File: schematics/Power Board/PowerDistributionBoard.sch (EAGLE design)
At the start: 11 parts

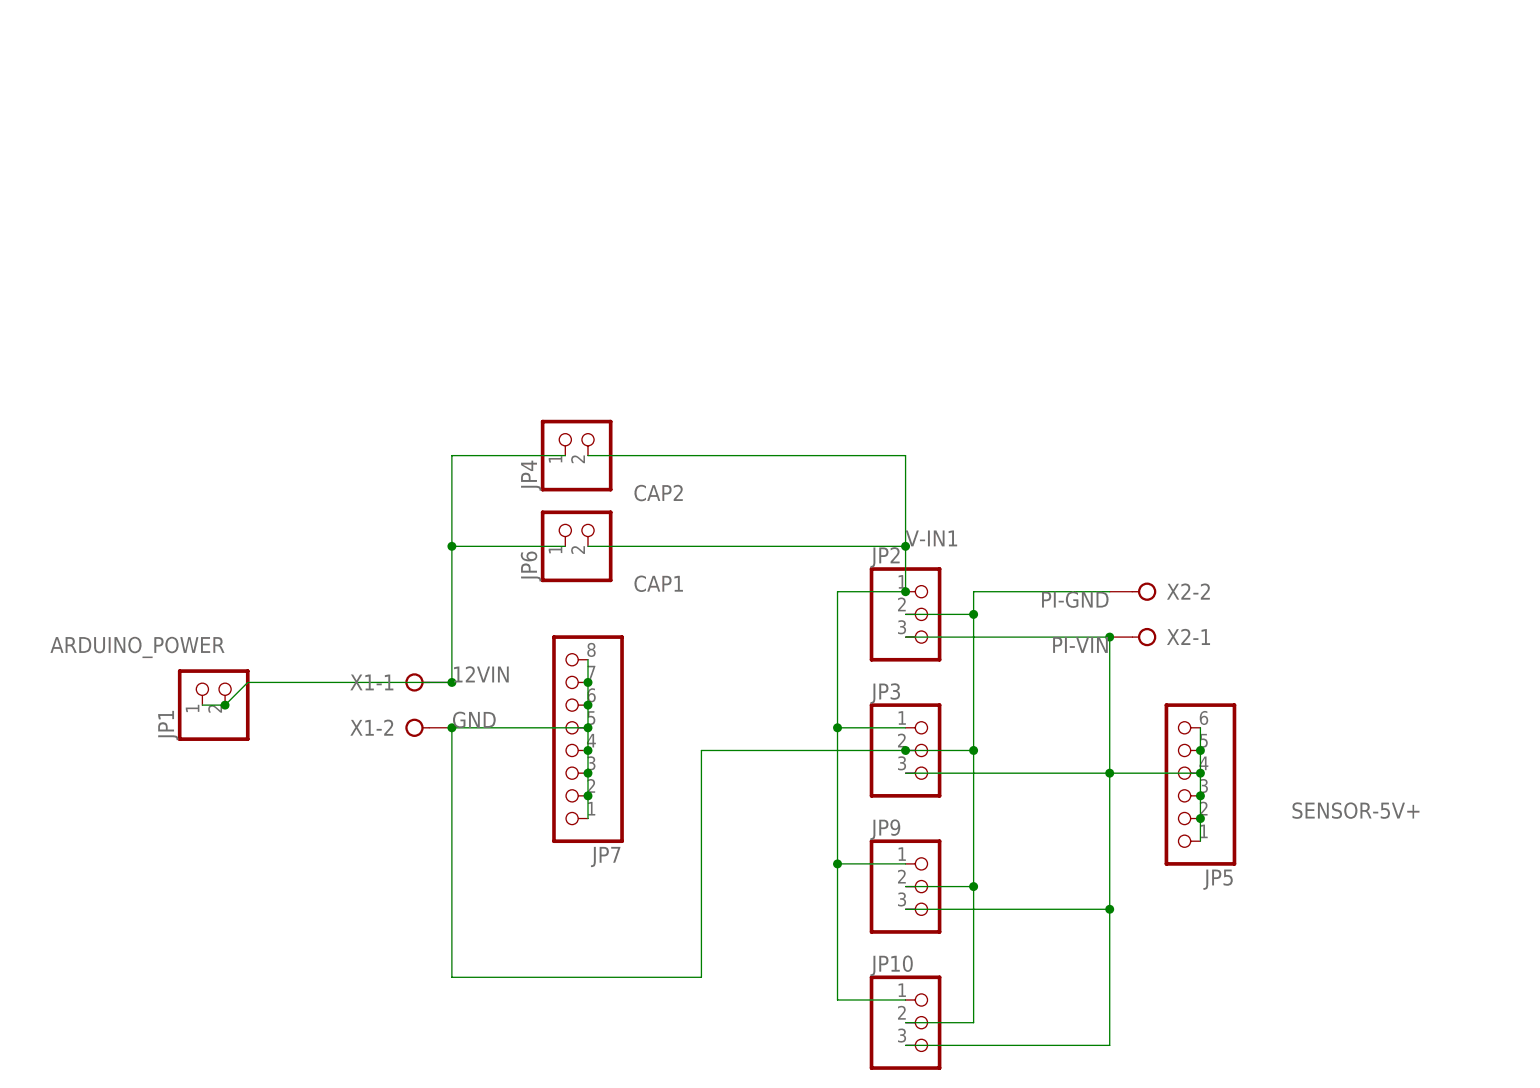
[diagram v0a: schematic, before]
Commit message: Updated Most Recent PCB's
Changed both directories with the most up to date schematics.
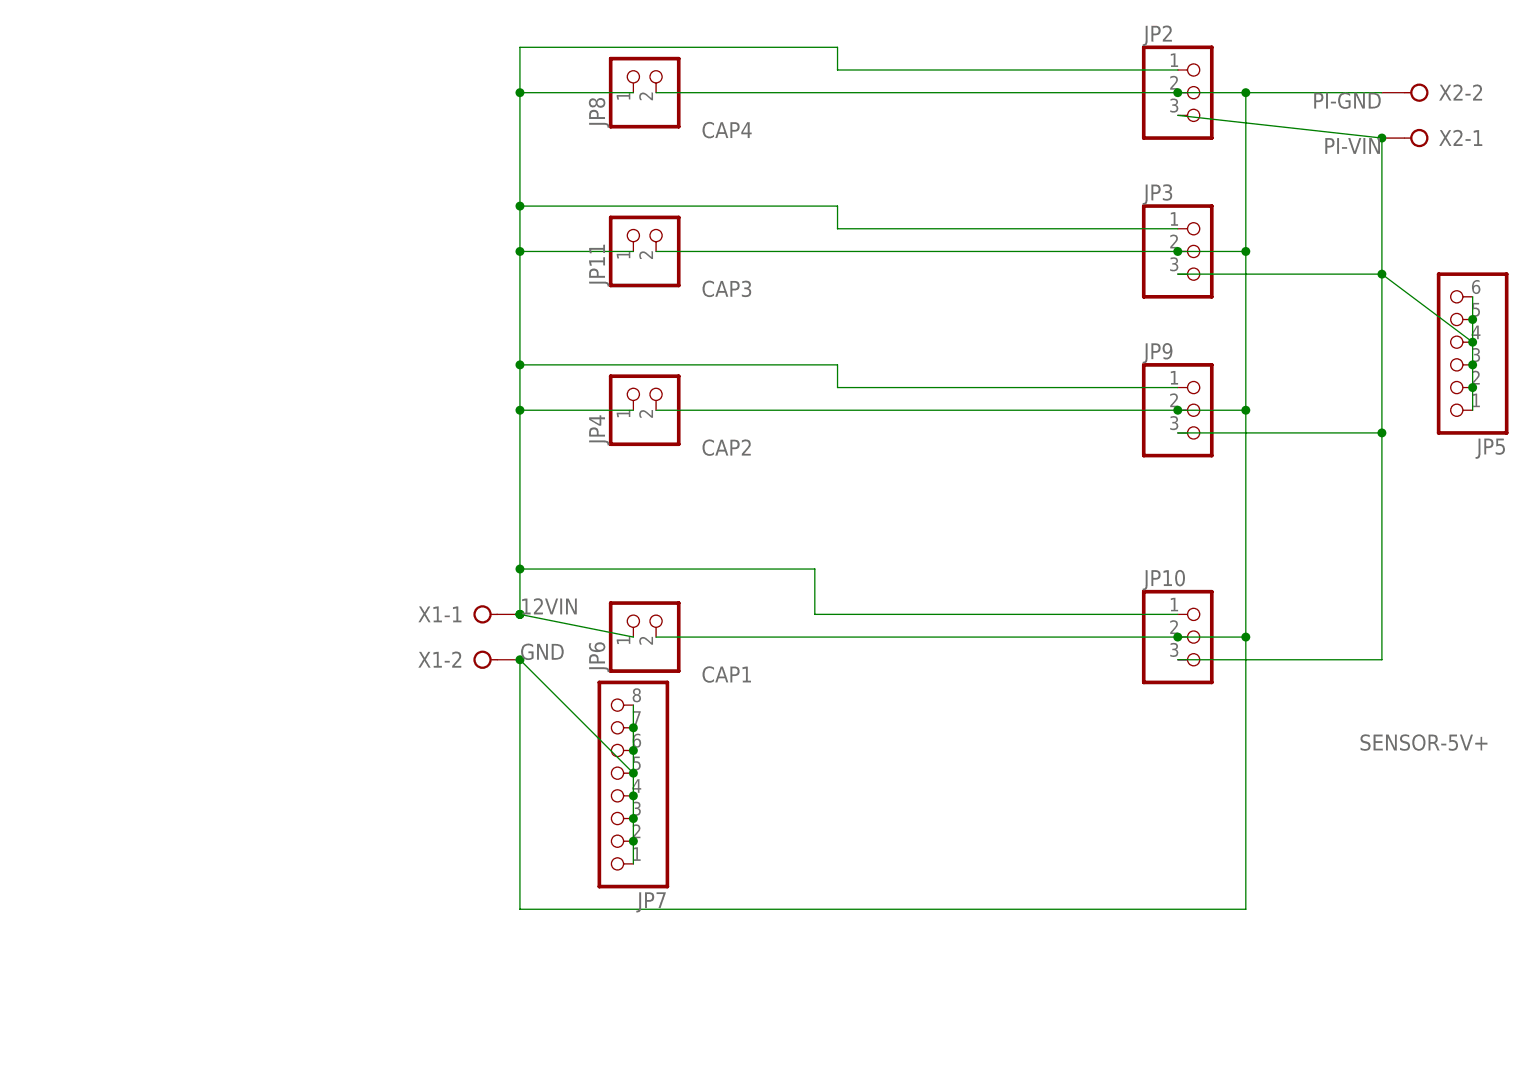
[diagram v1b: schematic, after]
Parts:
- removed JP1: (no value), pinhead:PINHD-1X2
- added JP11, JP8: (no value), pinhead:PINHD-1X2
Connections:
- removed net V-IN1: JP10.1, JP2.1, JP3.1, JP4.2, JP6.2, JP9.1
- net COMMON-GND: now also JP11.2, JP4.2, JP6.2, JP8.2
- net N$1: now also JP10.1, JP11.1, JP2.1, JP3.1, JP8.1, JP9.1; no longer JP1.1, JP1.2
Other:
- moved on the sheet: JP10, JP2, JP3, JP4, JP5, JP6, JP7, JP9, X1-1, X1-2, X2-1, X2-2
